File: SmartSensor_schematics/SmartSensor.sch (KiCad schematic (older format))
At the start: 50 parts, among them IC1 DS1337+, IC2 SHT31-DIS-B, IC3 VEML7700-TT, J1 ÉXTENSION HEADER, J3 Conn_02x04_Odd_Even, J4 FTDI cable connector, J6 Barrel_Jack, J8 6 PIN ISP, Q1 MMBF170, Q2 MMBF170, Q3 MMBF170, Q4 MMBF170, Q5 MMBF170, SW1 SW_Push, U1 AZ1117-3.3, U2 MCP9808_MSOP, U3 DMG2301l, U4 ATmega328P-AU, U5 XBee_SMT, U6 MCP1640BCH, X1 XTAL

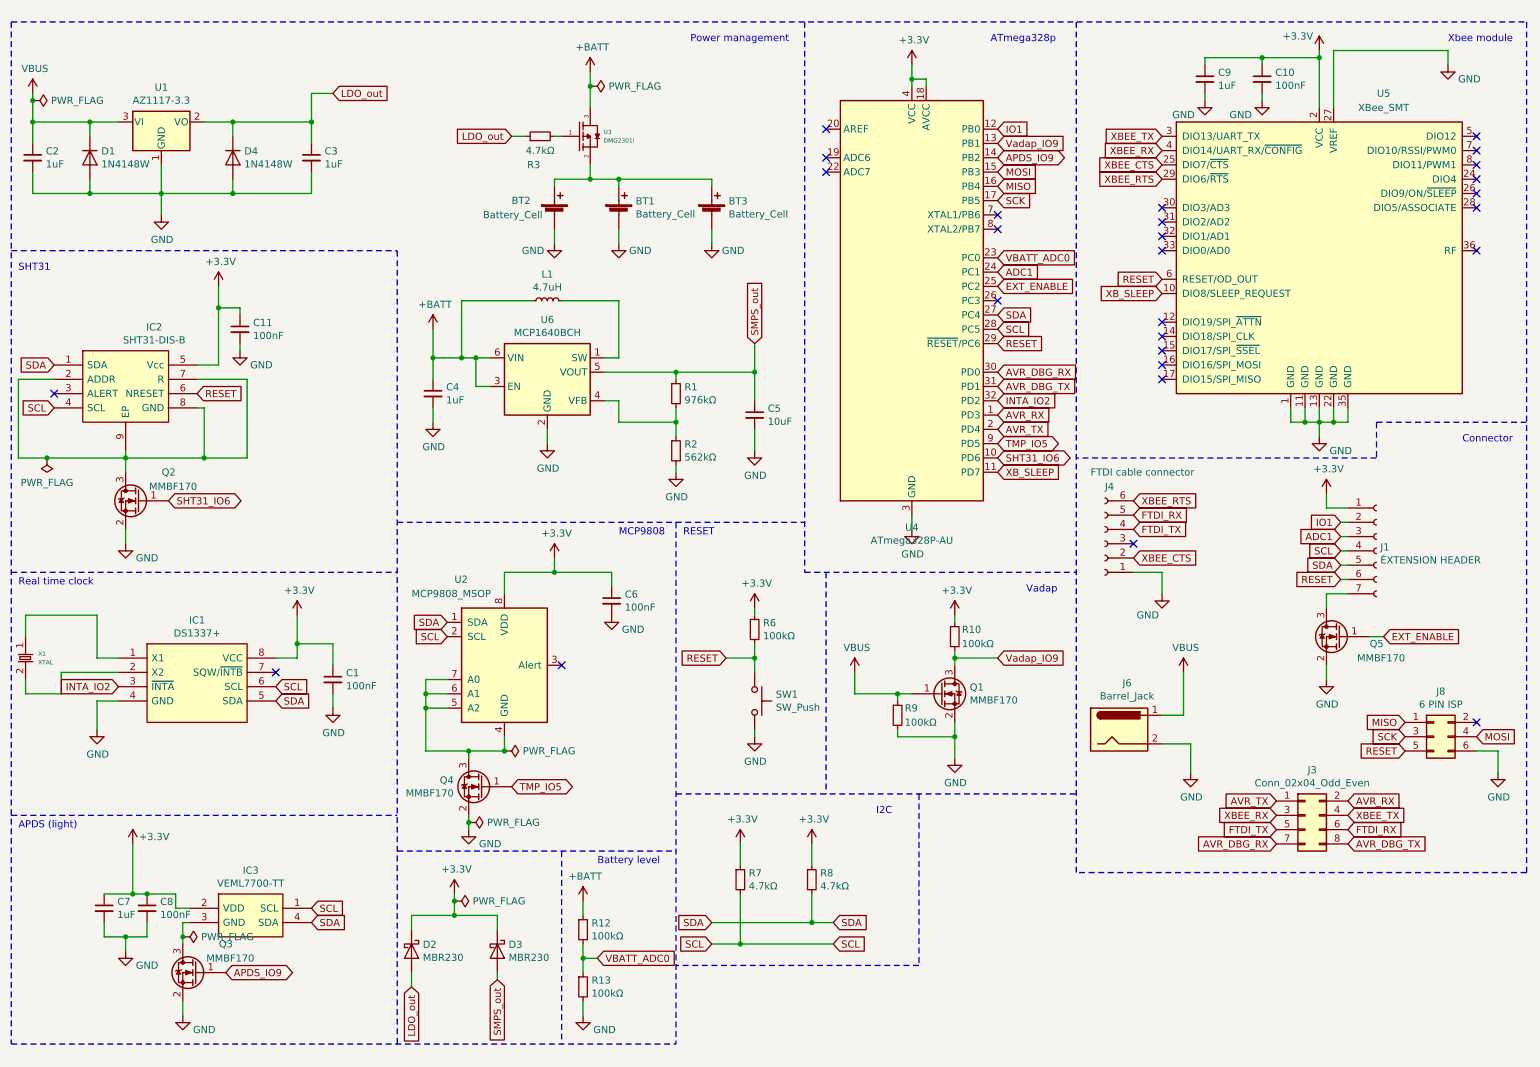
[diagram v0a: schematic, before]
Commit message: hardware: update hardware
Update the smart sensor hardware.

Signed-off-by: Michel Megens <michel@michelmegens.net>
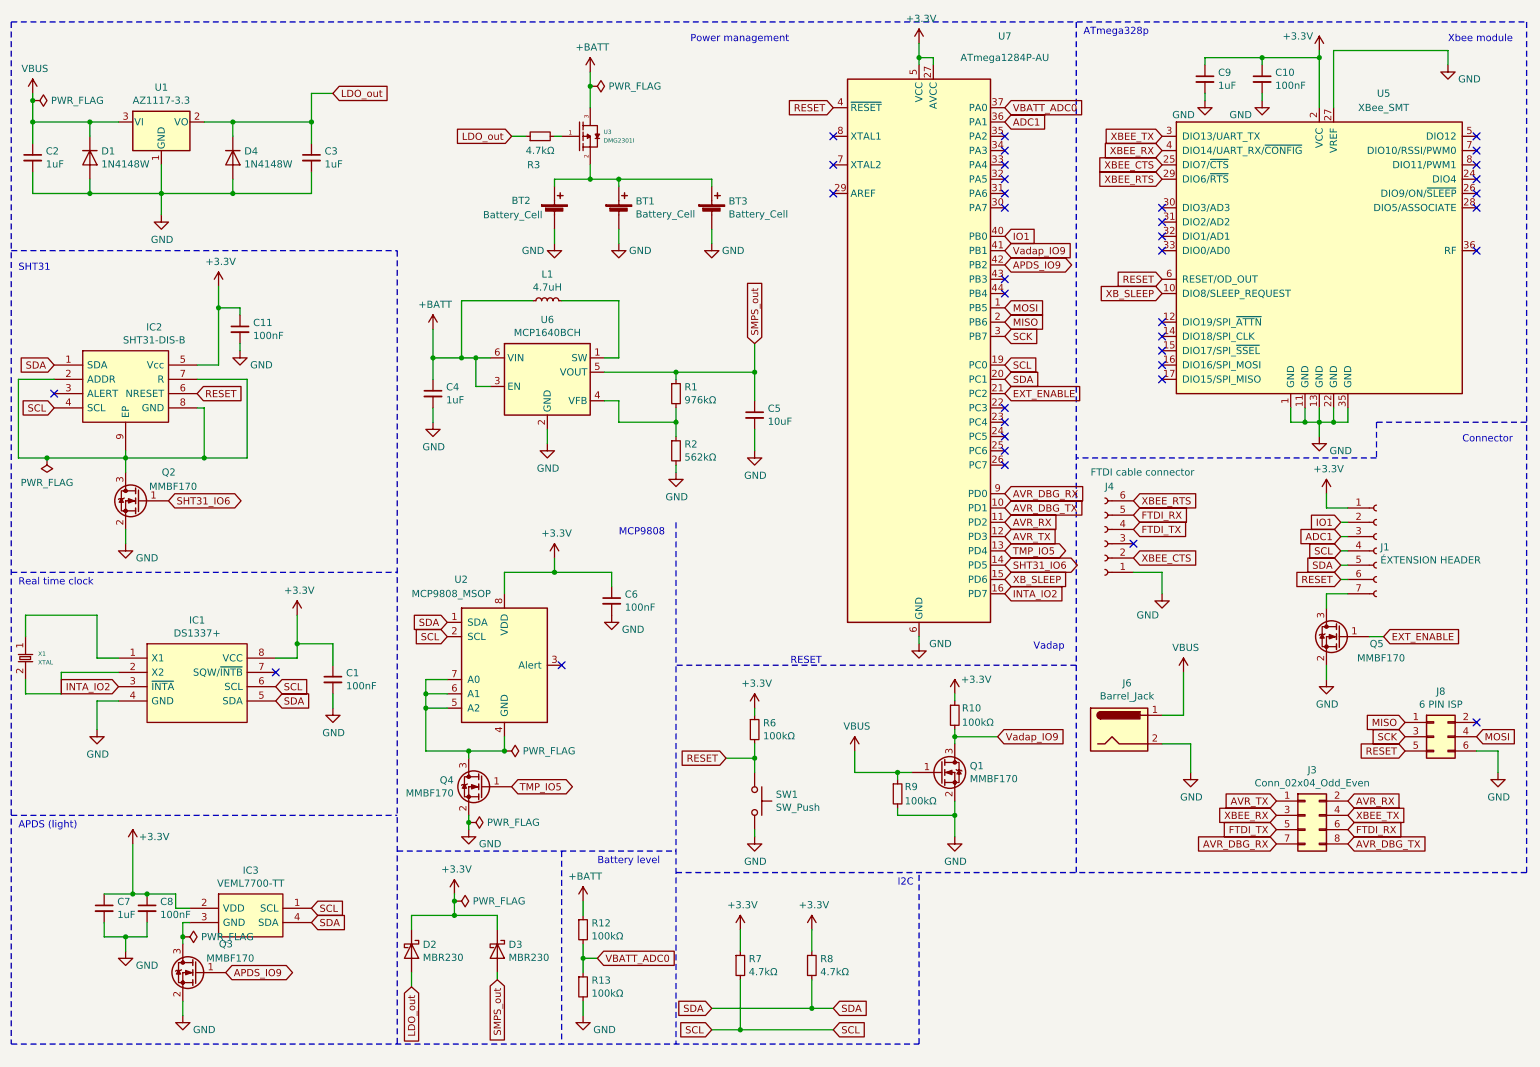
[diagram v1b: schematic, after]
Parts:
- removed U4: ATmega328P-AU, Package_QFP:TQFP-32_7x7mm_P0.8mm, symbol MCU_Microchip_ATmega:ATmega328P-AU
- added U7: ATmega1284P-AU, Package_QFP:TQFP-44_10x10mm_P0.8mm, symbol MCU_Microchip_ATmega:ATmega1284P-AU
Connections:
- net +3V3: now also U7.17 (VCC), U7.27 (AVCC), U7.38 (VCC), U7.5 (VCC)
- net ADC1: now also U7.36 (PA1)
- net APDS_IO9: now also U7.42 (PB2)
- net AVR_DBG_RX: now also U7.9 (PD0)
- net AVR_DBG_TX: now also U7.10 (PD1)
- net AVR_RX: now also U7.11 (PD2)
- net AVR_TX: now also U7.12 (PD3)
- net EXT_ENABLE: now also U7.21 (PC2)
- net GND: now also U7.18 (GND), U7.28 (GND), U7.39 (GND), U7.6 (GND)
- net INTA_IO2: now also U7.16 (PD7)
- net IO1: now also U7.40 (PB0)
- net MISO: now also U7.2 (PB6)
- net MOSI: now also U7.1 (PB5)
- net RESET: now also U7.4 (~RESET)
- net SCK: now also U7.3 (PB7)
- net SCL: now also U7.19 (PC0)
- net SDA: now also U7.20 (PC1)
- net SHT31_IO6: now also U7.14 (PD5)
- net TMP_IO5: now also U7.13 (PD4)
- net VBATT_ADC0: now also U7.37 (PA0)
- net Vadap_IO9: now also U7.41 (PB1)
- net XB_SLEEP: now also U7.15 (PD6)
- no-connect marks 27 -> 37
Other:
- moved on the sheet: Q1, R10, R6, R7, R8, R9, SW1
